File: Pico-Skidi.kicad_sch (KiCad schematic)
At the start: 10 parts, among them M1 Motor_DC, M2 Motor_DC, M3 Motor_DC, M4 Motor_Servo, M5 Motor_Servo, U1 Pico, U2 PDRV8411PWPR, U3 PDRV8411PWPR, U4 LM5156HPWPR

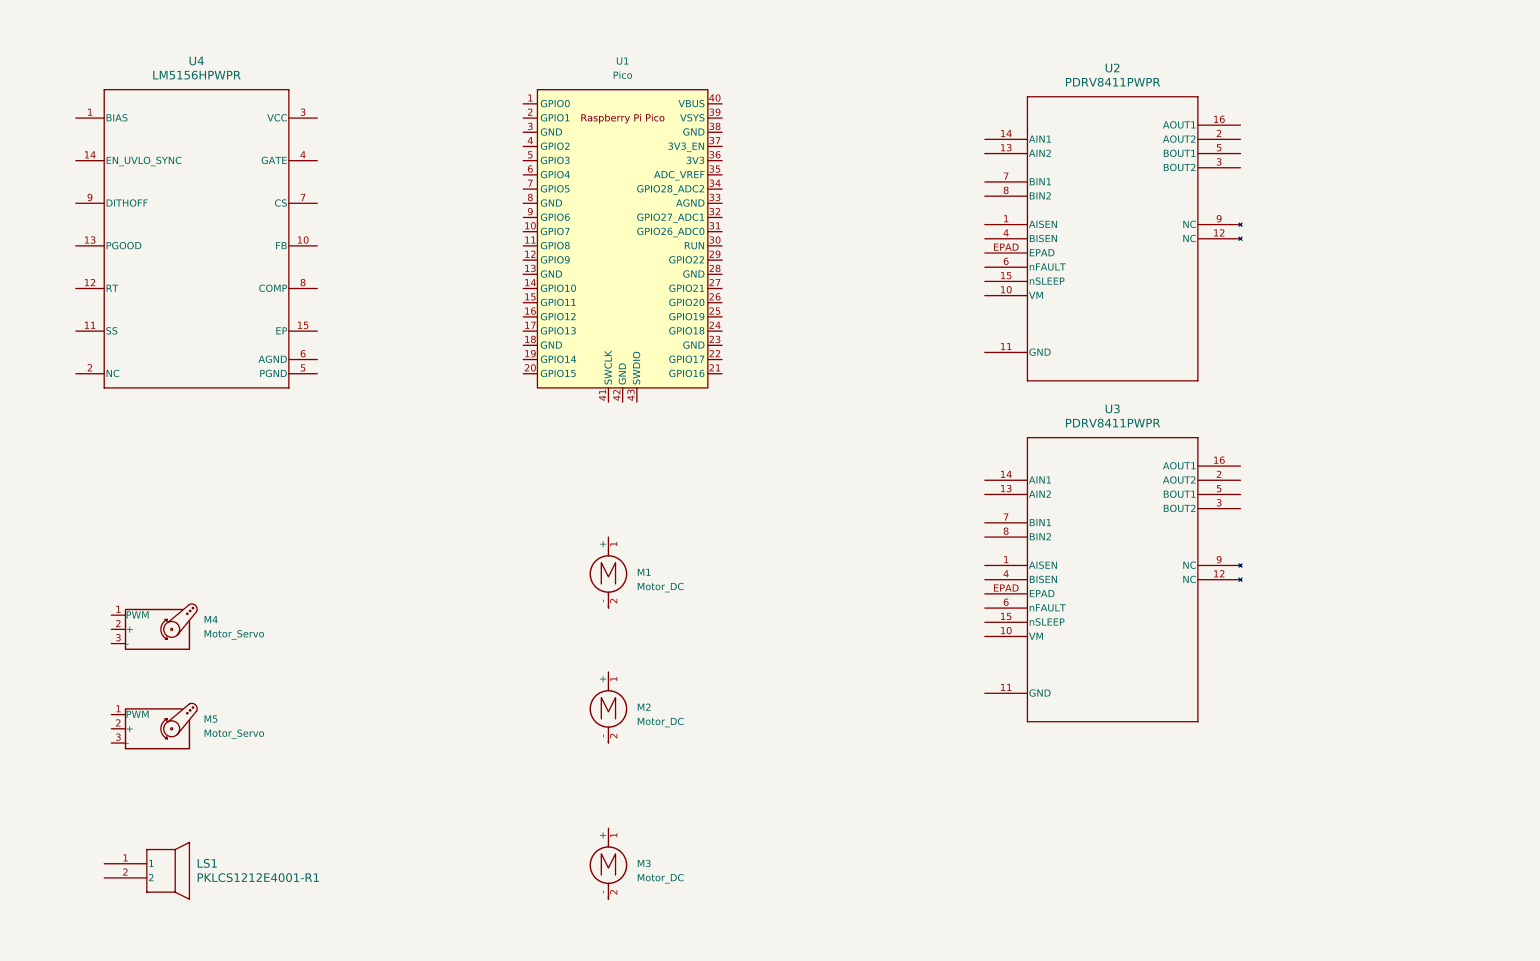
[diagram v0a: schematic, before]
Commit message: Starting on Power
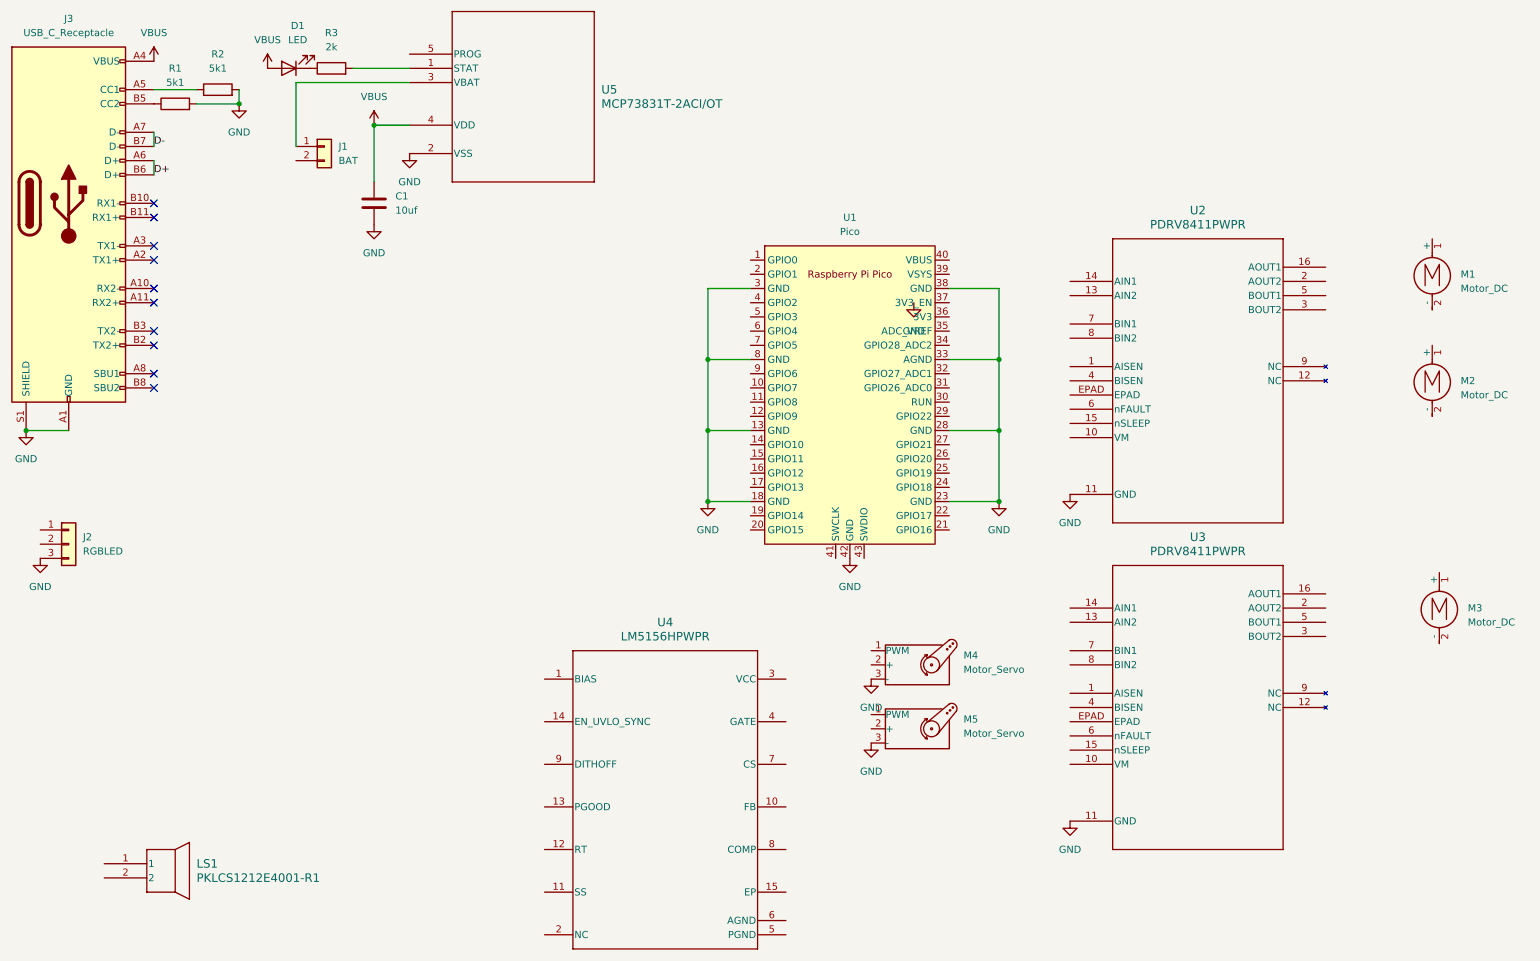
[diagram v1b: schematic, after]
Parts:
- added C1: 10uf, symbol Device:C
- added D1: LED, symbol Device:LED
- added J1: BAT, symbol Connector_Generic:Conn_01x02
- added J2: RGBLED, symbol Connector_Generic:Conn_01x03
- added J3: USB_C_Receptacle, symbol Connector:USB_C_Receptacle
- added R1, R2: 5k1, symbol Device:R
- added R3: 2k, symbol Device:R
- added U5: MCP73831T-2ACI/OT, SOT-23-5_MC_MCH, symbol MCP73831:MCP73831T-2ACI_OT
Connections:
- net GND: now reaches U2.11 (GND)
- net GND: now also M4.3 (-), M5.3 (-), U1.13 (GND), U1.18 (GND), U1.23 (GND), U1.28 (GND), U1.3 (GND), U1.33 (AGND), U1.38 (GND), U1.42 (GND), U1.8 (GND), U3.11 (GND), C1.2, J2.3 (Pin_3), J3.A1 (GND), J3.A12 (GND), J3.B1 (GND), J3.B12 (GND), J3.S1 (SHIELD), R1.2, R2.2, U5.2 (VSS)
- new net: D1.1 (K), R3.1
- new net: J3.A5 (CC1), R2.1
- new net: J3.B5 (CC2), R1.1
- new net: R3.2, U5.1 (STAT)
- new net: J1.1 (Pin_1), U5.3 (VBAT)
- new net D+: J3.A6 (D+), J3.B6 (D+)
- new net D-: J3.A7 (D-), J3.B7 (D-)
- new net VBUS: C1.1, D1.2 (A), J3.A4 (VBUS), J3.A9 (VBUS), J3.B4 (VBUS), J3.B9 (VBUS), U5.4 (VDD)
- no-connect marks 0 -> 10
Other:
- moved on the sheet: M1, M2, M3, M4, M5, U1, U2, U3, U4
